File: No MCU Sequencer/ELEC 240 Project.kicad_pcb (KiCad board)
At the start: 2 copper layers, 50.8 x 50.8 mm, 37 parts, among them Q4 NMOS, Q5 NMOS, Q6 NMOS, SW2 MODE, SW3 RECORD, SW7 Note1, SW8 Note2, SW9 Note3, U1 PLAYBACK, U2 74HC595, U3 74HC595, U4 74HC595, U6 TONEGEN, U9 RECORD

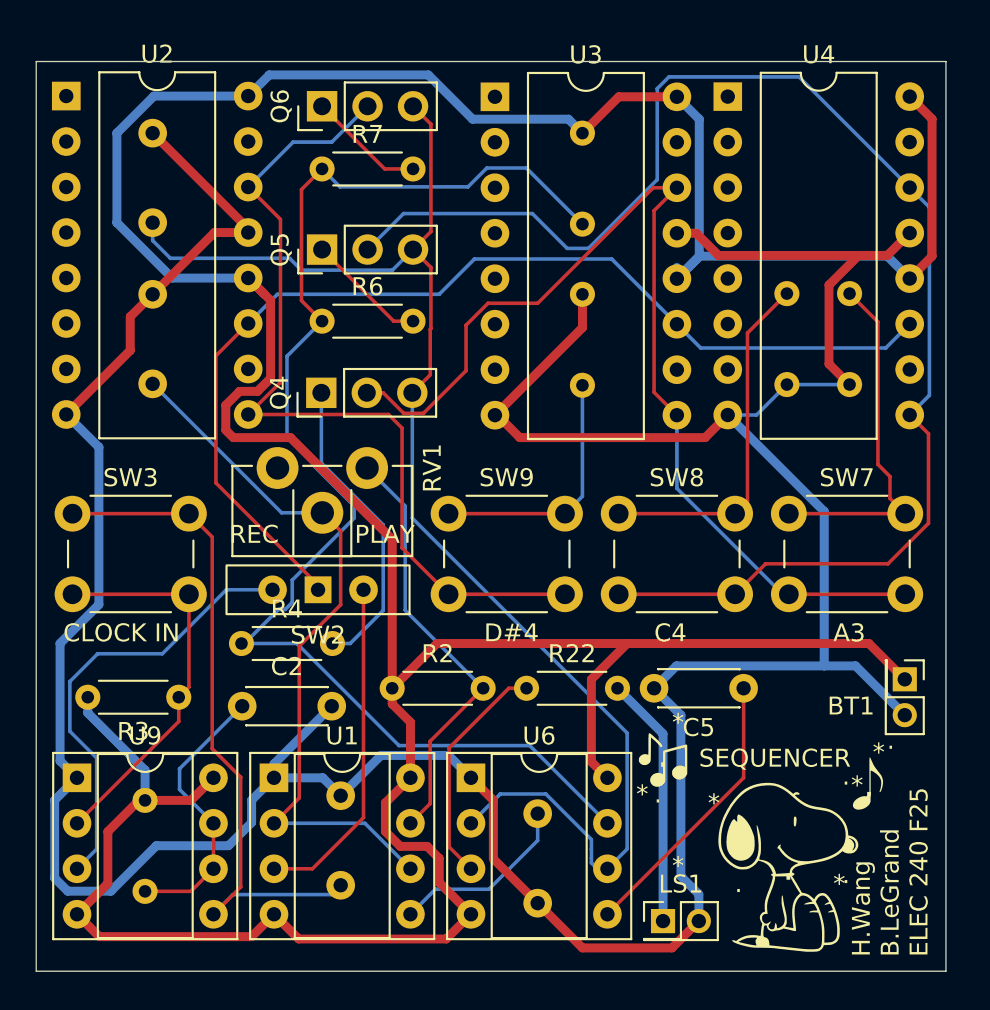
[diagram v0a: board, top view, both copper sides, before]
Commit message: Add files via upload
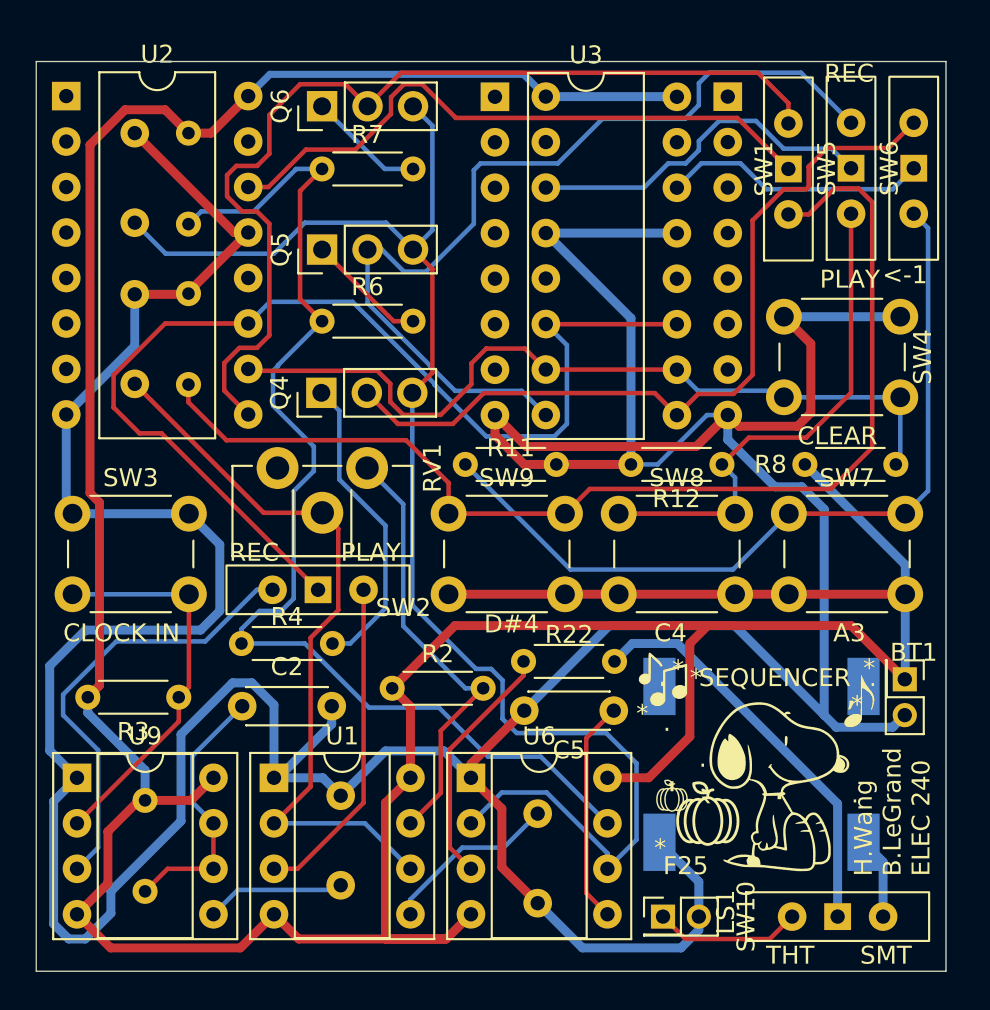
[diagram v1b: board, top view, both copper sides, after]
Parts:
- added ': LOGO, LOGO, F.Cu at (241.0, 83.5)
- added LS2: CDS-13138-SMT-TR, CDS-13138-SMT-TR:SPKR_CDS-13138-SMT-TR, B.Cu at (246.0, 81.8)
- added R8: 10k Ohms, Resistor_THT:R_Axial_DIN0204_L3.6mm_D1.6mm_P5.08mm_Horizontal, F.Cu at (248.4, 65.0)
- added SW1: MODE, Button_Switch_THT:SW_Slide-03_Wuerth-WS-SLTV_10x2.5x6.4_P2.54mm, F.Cu at (247.5, 48.5)
- added SW10: SPEAKER, Button_Switch_THT:SW_Slide-03_Wuerth-WS-SLTV_10x2.5x6.4_P2.54mm, F.Cu at (250.2, 90.2)
- added SW4: CLEAR, Button_Switch_THT:SW_PUSH_6mm, F.Cu at (247.2, 56.8)
- added SW5: MODE, Button_Switch_THT:SW_Slide-03_Wuerth-WS-SLTV_10x2.5x6.4_P2.54mm, F.Cu at (251.0, 48.5)
- added SW6: MODE, Button_Switch_THT:SW_Slide-03_Wuerth-WS-SLTV_10x2.5x6.4_P2.54mm, F.Cu at (254.5, 48.5)
- added `: LOGO, LOGO, F.Cu at (243.0, 84.5)
- C4: value 100uF -> 47uF
- R11, R12: value 1000 -> 10k Ohms; moved to F.Cu
- R13: value 1000 -> 10k Ohms
- R2: value 5.1k Ohms -> 15k Ohms
- U4: moved to B.Cu
- moved R11 23.5 mm to (229.5, 65.0), turned to 0 degrees
- moved R13 22.0 mm to (214.0, 60.5)
- moved R5 22.0 mm to (214.0, 46.5)
- moved R12 10.2 mm to (243.8, 65.0), turned to 180 degrees
- moved C5 7.36 mm to (237.8, 78.8)
- moved , 4.63 mm to (251.5, 78.2)
- moved . 4.53 mm to (247.0, 83.0)
- moved : 4.50 mm to (240.5, 77.0)
- moved R22 1.51 mm to (232.7, 76.0)
- moved C4 1.00 mm to (211.0, 60.5)
- moved C6 1.00 mm to (211.0, 51.5)
- moved LS1 0.25 mm to (240.5, 90.2)
- turned U4 to 180 degrees
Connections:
- LS1 pad 1: Net-(LS1-Pad1) -> Net-(SW10-C)
- R22 pad 2: Net-(LS1-Pad1) -> Net-(SW10-B)
- SW3 pad 1: Net-(U9-CV) -> GND
- SW7 pad 2: tone1 -> +5V
- SW8 pad 2: tone2 -> +5V
- SW9 pad 2: tone3 -> +5V
- U2 pad 10: unconnected-(U2-~{SRCLR}-Pad10) -> CLR
- U2 pad 12: +5V -> unconnected-(U2-RCLK-Pad12)
- U2 pad 14: tone3 -> Net-(SW1-B)
- U3 pad 10: unconnected-(U3-~{SRCLR}-Pad10) -> CLR
- U3 pad 12: +5V -> unconnected-(U3-RCLK-Pad12)
- U3 pad 14: tone1 -> Net-(SW6-B)
- U4 pad 10: unconnected-(U4-~{SRCLR}-Pad10) -> CLR
- U4 pad 12: +5V -> unconnected-(U4-RCLK-Pad12)
- U4 pad 14: tone2 -> Net-(SW5-B)
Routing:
- net GND: track 205.4 -> 260.9 mm
- net Net-(SW1-C): track 14.1 -> 63.6 mm
- net CLR: track 0.00 -> 45.3 mm
- net Net-(SW1-B): track 0.00 -> 35.1 mm
- net Net-(U9-CV): track 38.5 -> 7.78 mm
- net tone2: track 80.5 -> 51.3 mm
- net Net-(SW6-C): track 20.1 -> 45.9 mm
- net Net-(SW10-B): track 0.00 -> 22.9 mm
- net Net-(SW5-B): track 0.00 -> 20.0 mm
- net Net-(SW6-B): track 0.00 -> 14.9 mm
- net Net-(LS1-Pad1): track 14.1 -> 0.00 mm
- net tone1: track 57.5 -> 45.0 mm
- net Net-(SW5-C): track 20.0 -> 28.4 mm
- net Net-(U6-DIS): track 73.6 -> 65.3 mm
- net Net-(SW10-C): track 0.00 -> 8.25 mm
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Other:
- board text added: "<-1"
- board text added: "CLEAR"
- board text added: "F25"
- board text added: "H.Wang B.LeGrand ELEC 240"
- board text added: "SMT"
- board text added: "THT"
- board text removed: "H.Wang B.LeGrand ELEC 240 F25"
